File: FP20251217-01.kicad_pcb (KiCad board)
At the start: 2 copper layers, 1 part, among them J1 216-3340-00-0602J

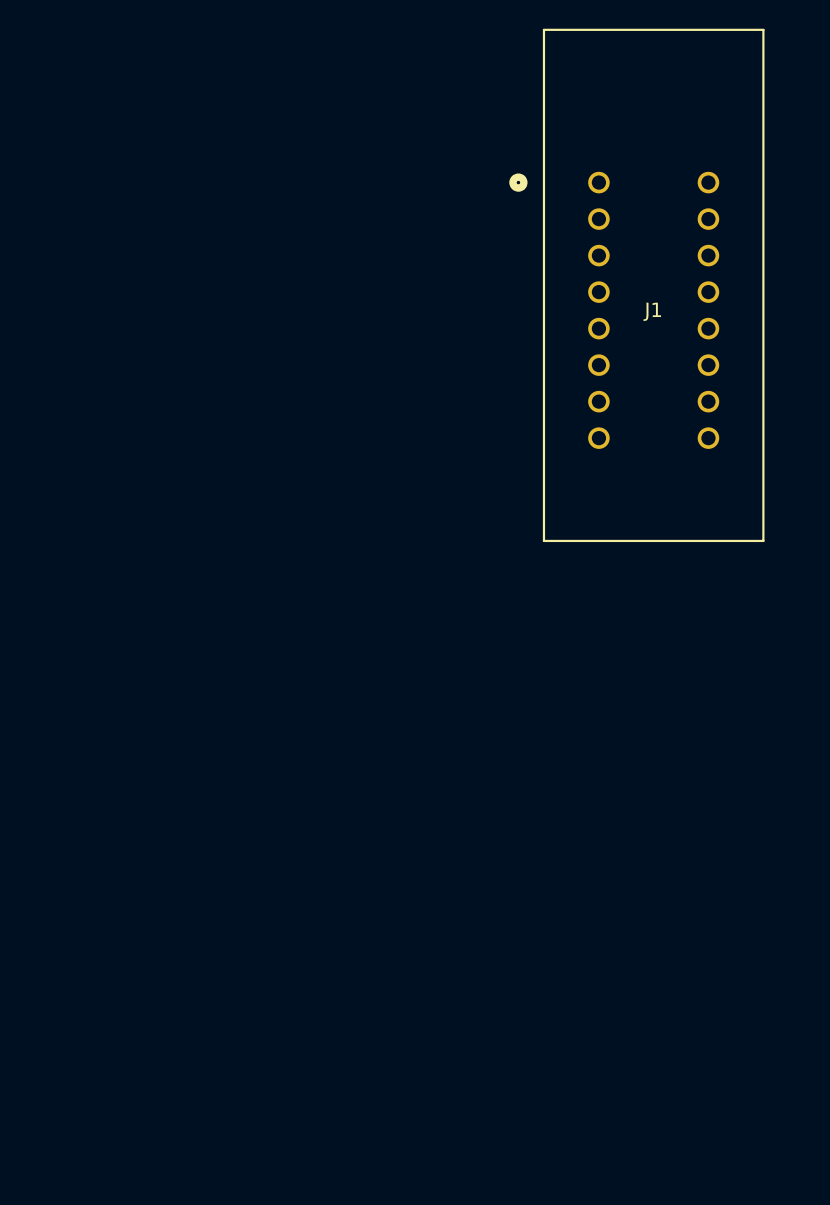
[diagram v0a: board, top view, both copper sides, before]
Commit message: Roughing out PCB
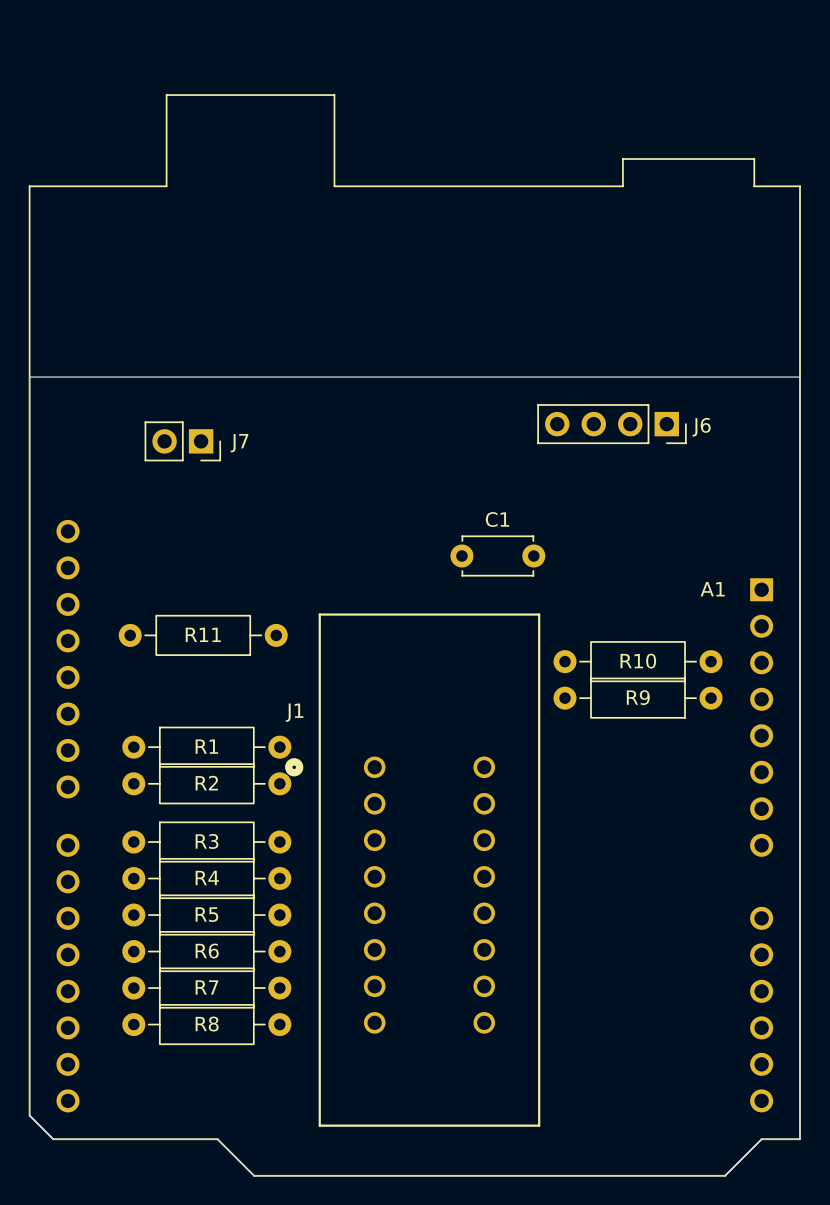
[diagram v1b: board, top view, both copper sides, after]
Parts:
- added A1: Arduino_UNO_R2, Module:Arduino_UNO_R2, F.Cu at (150.0, 100.0)
- added C1: 0.1u, Capacitor_THT:C_Disc_D4.7mm_W2.5mm_P5.00mm, F.Cu at (129.2, 97.7)
- added J6: Display, Connector_PinSocket_2.54mm:PinSocket_1x04_P2.54mm_Vertical, F.Cu at (143.4, 88.5)
- added J7: Read Button, Connector_PinSocket_2.54mm:PinSocket_1x02_P2.54mm_Vertical, F.Cu at (111.0, 89.7)
- added R1: 10k, Resistor_THT:R_Axial_DIN0207_L6.3mm_D2.5mm_P10.16mm_Horizontal, F.Cu at (106.3, 111.0)
- added R10: 10k, Resistor_THT:R_Axial_DIN0207_L6.3mm_D2.5mm_P10.16mm_Horizontal, F.Cu at (146.5, 105.0)
- added R11: 10k, Resistor_THT:R_Axial_DIN0207_L6.3mm_D2.5mm_P10.16mm_Horizontal, F.Cu at (116.2, 103.2)
- added R2: 10k, Resistor_THT:R_Axial_DIN0207_L6.3mm_D2.5mm_P10.16mm_Horizontal, F.Cu at (106.3, 113.5)
- added R3: 10k, Resistor_THT:R_Axial_DIN0207_L6.3mm_D2.5mm_P10.16mm_Horizontal, F.Cu at (106.3, 117.5)
- added R4: 10k, Resistor_THT:R_Axial_DIN0207_L6.3mm_D2.5mm_P10.16mm_Horizontal, F.Cu at (106.3, 120.1)
- added R5: 10k, Resistor_THT:R_Axial_DIN0207_L6.3mm_D2.5mm_P10.16mm_Horizontal, F.Cu at (106.3, 122.6)
- added R6: 10k, Resistor_THT:R_Axial_DIN0207_L6.3mm_D2.5mm_P10.16mm_Horizontal, F.Cu at (106.3, 125.2)
- added R7: 10k, Resistor_THT:R_Axial_DIN0207_L6.3mm_D2.5mm_P10.16mm_Horizontal, F.Cu at (106.3, 127.7)
- added R8: 10k, Resistor_THT:R_Axial_DIN0207_L6.3mm_D2.5mm_P10.16mm_Horizontal, F.Cu at (106.3, 130.2)
- added R9: 10k, Resistor_THT:R_Axial_DIN0207_L6.3mm_D2.5mm_P10.16mm_Horizontal, F.Cu at (146.5, 107.5)
- moved J1 43.6 mm to (123.1, 112.3)
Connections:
- J1 pad 1: unconnected-(J1-Pad1) -> /O1
- J1 pad 10: unconnected-(J1-Pad10) -> /A0
- J1 pad 11: unconnected-(J1-Pad11) -> /A1
- J1 pad 12: unconnected-(J1-Pad12) -> /A2
- J1 pad 13: unconnected-(J1-Pad13) -> /A3
- J1 pad 14: unconnected-(J1-Pad14) -> /A4
- J1 pad 15: unconnected-(J1-Pad15) -> /~{CE}
- J1 pad 16: unconnected-(J1-Pad16) -> +5V
- J1 pad 2: unconnected-(J1-Pad2) -> /O2
- J1 pad 3: unconnected-(J1-Pad3) -> /O3
- J1 pad 4: unconnected-(J1-Pad4) -> /O4
- J1 pad 5: unconnected-(J1-Pad5) -> /O5
- J1 pad 6: unconnected-(J1-Pad6) -> /O6
- J1 pad 7: unconnected-(J1-Pad7) -> /O7
- J1 pad 8: unconnected-(J1-Pad8) -> GND
- J1 pad 9: unconnected-(J1-Pad9) -> /O8
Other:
- board outline added: 53.6 x 55.6 mm
